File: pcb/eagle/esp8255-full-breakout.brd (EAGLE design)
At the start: 23.4 x 35 mm, 12 parts, among them IC1 ESP-12E/F, X1 JST-XH-11-PIN-ROUND-PAD, X2 JST-XH-11-PIN-ROUND-PAD

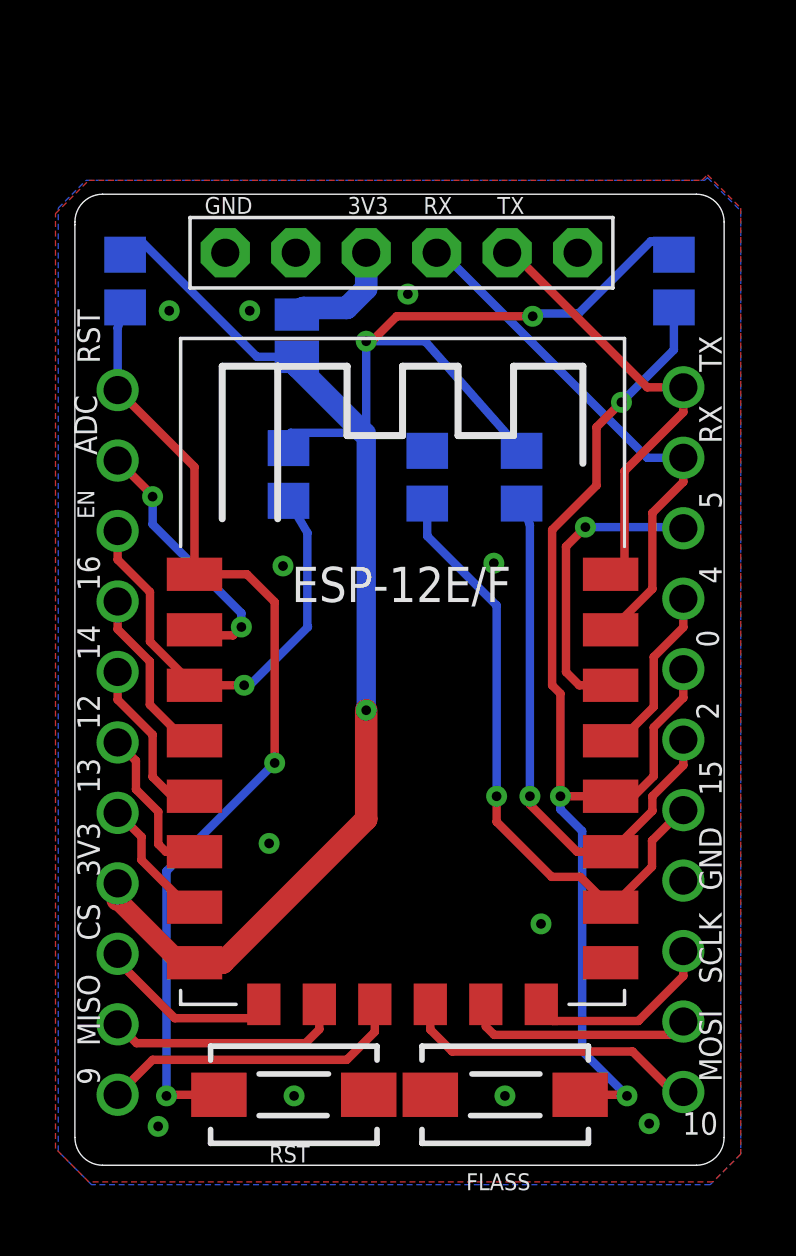
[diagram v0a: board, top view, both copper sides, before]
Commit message: Version 1.1
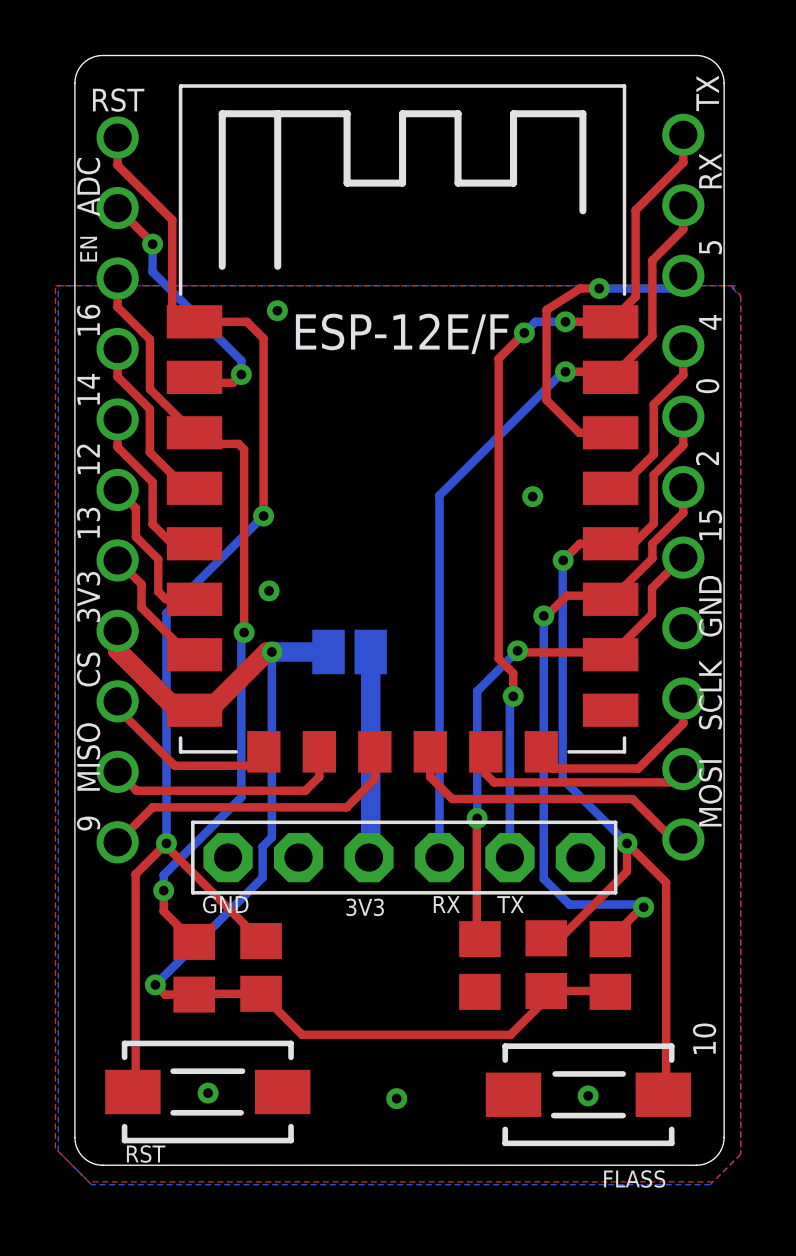
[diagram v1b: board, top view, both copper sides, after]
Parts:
- moved R1 25.2 mm to (6.71, 7.13), flipped to the top, turned to 90 degrees
- moved R2 25.1 mm to (17.0, 7.23), flipped to the top, turned to 90 degrees
- moved JP1 21.8 mm to (11.9, 11.1)
- moved R5 18.1 mm to (4.30, 7.10), flipped to the top, turned to 90 degrees
- moved R4 17.9 mm to (19.3, 7.20), flipped to the top, turned to 90 degrees
- moved R3 17.7 mm to (14.6, 7.20), flipped to the top, turned to 270 degrees
- moved SJ1 11.6 mm to (9.90, 18.5), turned to 180 degrees
- moved IC1 9.10 mm to (11.8, 22.9)
- moved X2 9.10 mm to (21.9, 24.4)
- moved X1 9.10 mm to (1.54, 24.3)
- moved S1 3.10 mm to (4.79, 2.64)
- moved S2 3.00 mm to (18.5, 2.54)
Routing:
- net +3V3: track 65.4 -> 41.8 mm, vias 3 -> 2
- net TXD: track 16.2 -> 30.7 mm, vias 0 -> 3
- net EN: track 16.4 -> 28.2 mm, vias 1 -> 2
- net RST: track 35.4 -> 44.8 mm
- net RXD: track 19.3 -> 28.5 mm, vias 0 -> 1
- net IO0: track 41.0 -> 33.9 mm, vias 3 -> 2
- net IO2: track 19.7 -> 23.2 mm, vias 1 -> 2
- net IO15: track 22.5 -> 19.1 mm, vias 1 -> 2
- net N$1: track 4.18 -> 7.44 mm
- net IO5: track 10.9 -> 11.4 mm
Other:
- board size 23.4 x 35 mm -> 23.4 x 40 mm
- board text added: "Rev.1.1 (C) 2020"
- board text removed: "Rev.1.0 (C) 2020"
